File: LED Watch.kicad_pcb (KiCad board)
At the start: 2 copper layers, 41.9 x 49.3 mm, 140 parts, among them J1 AVR-ISP-6, J2 Lipo, J3 Coin Cell, SW1 SW_DPST, SW2 SW_DPST, U10 B39D3RGB-F6C0001HOU1930, U100 B39D3RGB-F6C0001HOU1930, U101 B39D3RGB-F6C0001HOU1930, U102 B39D3RGB-F6C0001HOU1930, U103 B39D3RGB-F6C0001HOU1930, U104 B39D3RGB-F6C0001HOU1930, U105 B39D3RGB-F6C0001HOU1930, U106 B39D3RGB-F6C0001HOU1930, U107 B39D3RGB-F6C0001HOU1930, U108 B39D3RGB-F6C0001HOU1930, U109 B39D3RGB-F6C0001HOU1930, U11 B39D3RGB-F6C0001HOU1930, U110 B39D3RGB-F6C0001HOU1930, U111 B39D3RGB-F6C0001HOU1930, U112 B39D3RGB-F6C0001HOU1930, U113 B39D3RGB-F6C0001HOU1930, U114 B39D3RGB-F6C0001HOU1930, U115 B39D3RGB-F6C0001HOU1930, U116 B39D3RGB-F6C0001HOU1930, U117 B39D3RGB-F6C0001HOU1930, U118 B39D3RGB-F6C0001HOU1930, U119 B39D3RGB-F6C0001HOU1930, U12 B39D3RGB-F6C0001HOU1930, U120 B39D3RGB-F6C0001HOU1930, U121 B39D3RGB-F6C0001HOU1930, U122 B39D3RGB-F6C0001HOU1930, U123 B39D3RGB-F6C0001HOU1930, U124 B39D3RGB-F6C0001HOU1930, U125 B39D3RGB-F6C0001HOU1930, U126 B39D3RGB-F6C0001HOU1930, U127 B39D3RGB-F6C0001HOU1930, U128 B39D3RGB-F6C0001HOU1930, U129 B39D3RGB-F6C0001HOU1930, U13 B39D3RGB-F6C0001HOU1930, U130 B39D3RGB-F6C0001HOU1930, U131 B39D3RGB-F6C0001HOU1930, U132 B39D3RGB-F6C0001HOU1930, U133 B39D3RGB-F6C0001HOU1930, U134 BMI160, U135 ATmega165PA-M, U14 B39D3RGB-F6C0001HOU1930, U15 B39D3RGB-F6C0001HOU1930, U16 B39D3RGB-F6C0001HOU1930, U17 B39D3RGB-F6C0001HOU1930, U18 B39D3RGB-F6C0001HOU1930, U19 B39D3RGB-F6C0001HOU1930, U2 B39D3RGB-F6C0001HOU1930, U20 B39D3RGB-F6C0001HOU1930, U21 B39D3RGB-F6C0001HOU1930, U22 B39D3RGB-F6C0001HOU1930, U23 B39D3RGB-F6C0001HOU1930, U24 B39D3RGB-F6C0001HOU1930, U25 B39D3RGB-F6C0001HOU1930, U26 B39D3RGB-F6C0001HOU1930, U27 B39D3RGB-F6C0001HOU1930, U28 B39D3RGB-F6C0001HOU1930, U29 B39D3RGB-F6C0001HOU1930, U3 B39D3RGB-F6C0001HOU1930, U30 B39D3RGB-F6C0001HOU1930, U31 B39D3RGB-F6C0001HOU1930, U32 B39D3RGB-F6C0001HOU1930, U33 B39D3RGB-F6C0001HOU1930, U34 B39D3RGB-F6C0001HOU1930, U35 B39D3RGB-F6C0001HOU1930, U36 B39D3RGB-F6C0001HOU1930, U37 B39D3RGB-F6C0001HOU1930, U38 B39D3RGB-F6C0001HOU1930, U39 B39D3RGB-F6C0001HOU1930, U4 B39D3RGB-F6C0001HOU1930, U40 B39D3RGB-F6C0001HOU1930, U41 B39D3RGB-F6C0001HOU1930, U42 B39D3RGB-F6C0001HOU1930, U43 B39D3RGB-F6C0001HOU1930, U44 B39D3RGB-F6C0001HOU1930, U45 B39D3RGB-F6C0001HOU1930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

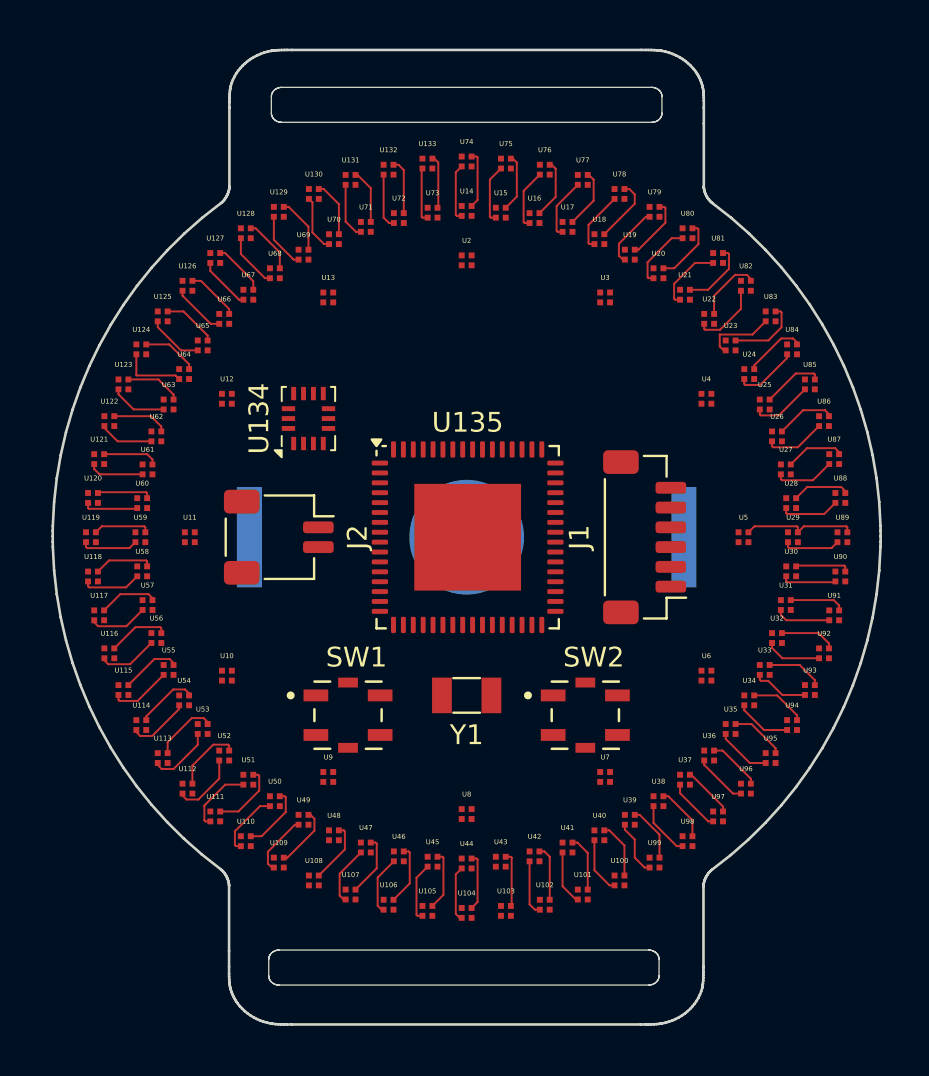
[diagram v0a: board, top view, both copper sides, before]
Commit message: added caps.. still unsuccessful routing
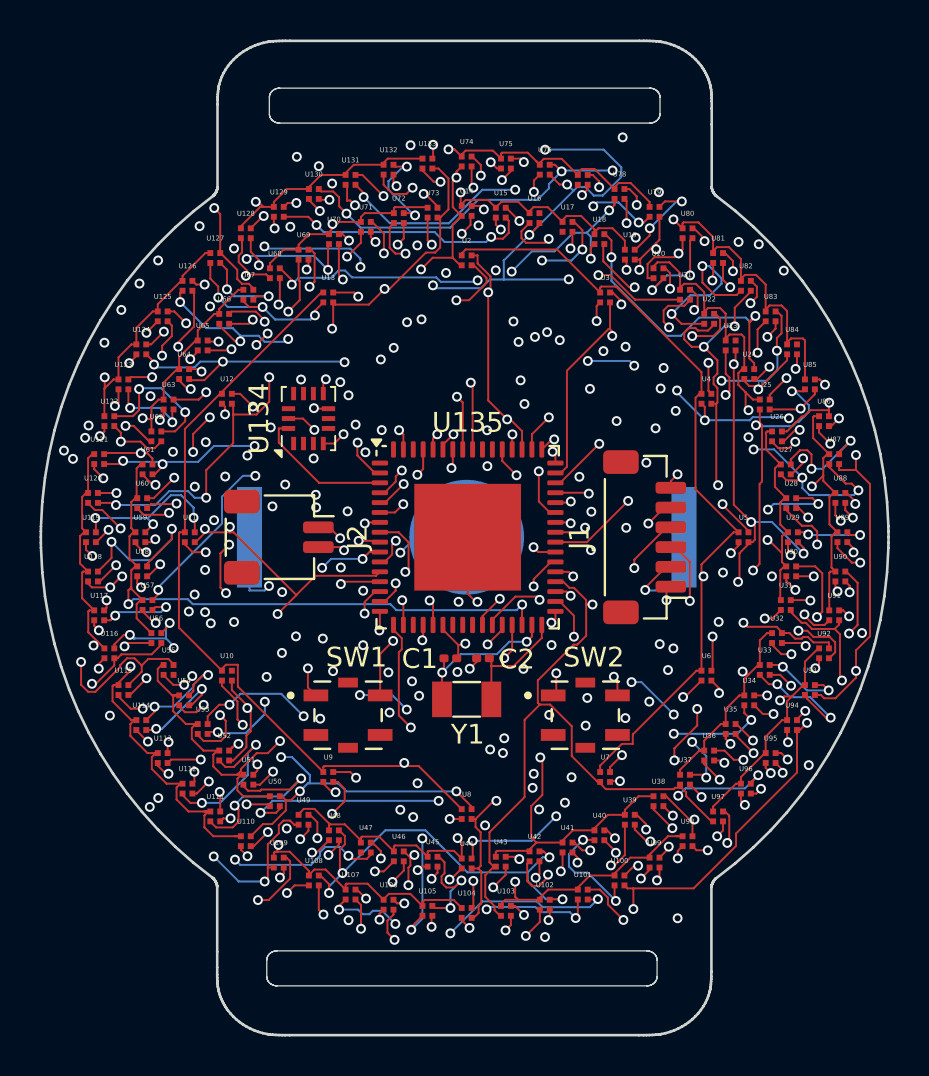
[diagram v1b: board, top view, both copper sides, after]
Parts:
- added C1: C, Capacitor_SMD:C_0201_0603Metric, F.Cu at (99.2, 106.1)
- added C2: C, Capacitor_SMD:C_0201_0603Metric, F.Cu at (100.8, 106.1)
- moved Y1 0.20 mm to (100.0, 108.2)
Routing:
- net /G3: track 0.00 -> 199.2 mm, vias 0 -> 31
- net /G5: track 0.00 -> 194.5 mm, vias 0 -> 33
- net /G2: track 0.00 -> 190.8 mm, vias 0 -> 32
- net /G6: track 0.00 -> 187.2 mm, vias 0 -> 27
- net /G1: track 0.00 -> 182.5 mm, vias 0 -> 26
- net /G4: track 0.00 -> 176.7 mm, vias 0 -> 32
- net /R6: track 28.8 -> 203.0 mm, vias 0 -> 28
- net /B3: track 30.7 -> 203.0 mm, vias 0 -> 36
- net /R5: track 29.1 -> 200.8 mm, vias 0 -> 34
- net /B2: track 30.3 -> 201.3 mm, vias 0 -> 31
- net /B5: track 25.9 -> 187.7 mm, vias 0 -> 33
- net /R4: track 32.9 -> 193.0 mm, vias 0 -> 32
- net /R2: track 30.2 -> 187.7 mm, vias 0 -> 29
- net /B6: track 26.2 -> 183.1 mm, vias 0 -> 25
- net /B1: track 29.7 -> 179.1 mm, vias 0 -> 26
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- added copper zone on In1.Cu, net Net-(J1-GND)
- added copper zone on In2.Cu, net Net-(J1-VCC)
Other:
- board size 41.9 x 49.3 mm -> 42.9 x 50.3 mm
- copper layers 2 -> 4
